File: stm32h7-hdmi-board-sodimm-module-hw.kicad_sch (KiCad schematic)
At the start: 8 parts

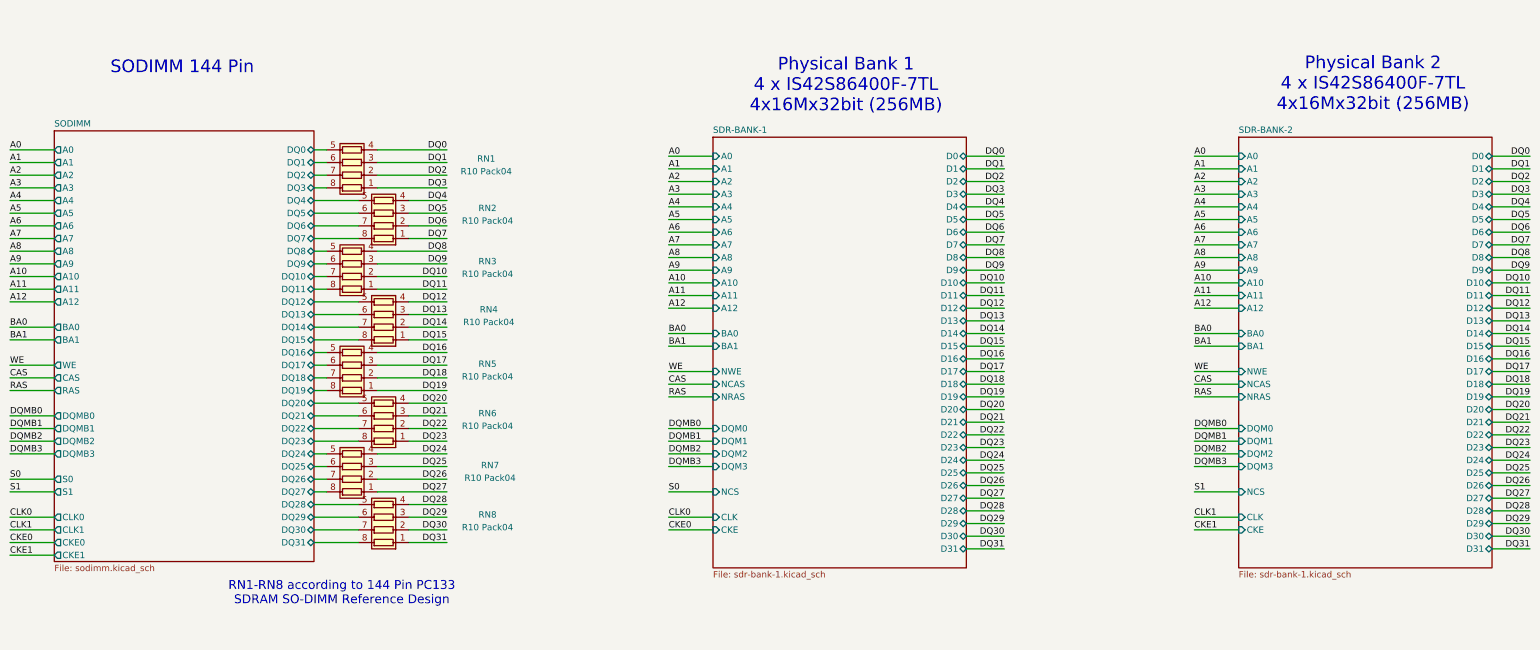
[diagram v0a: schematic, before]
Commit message: [#100470] Update schematic
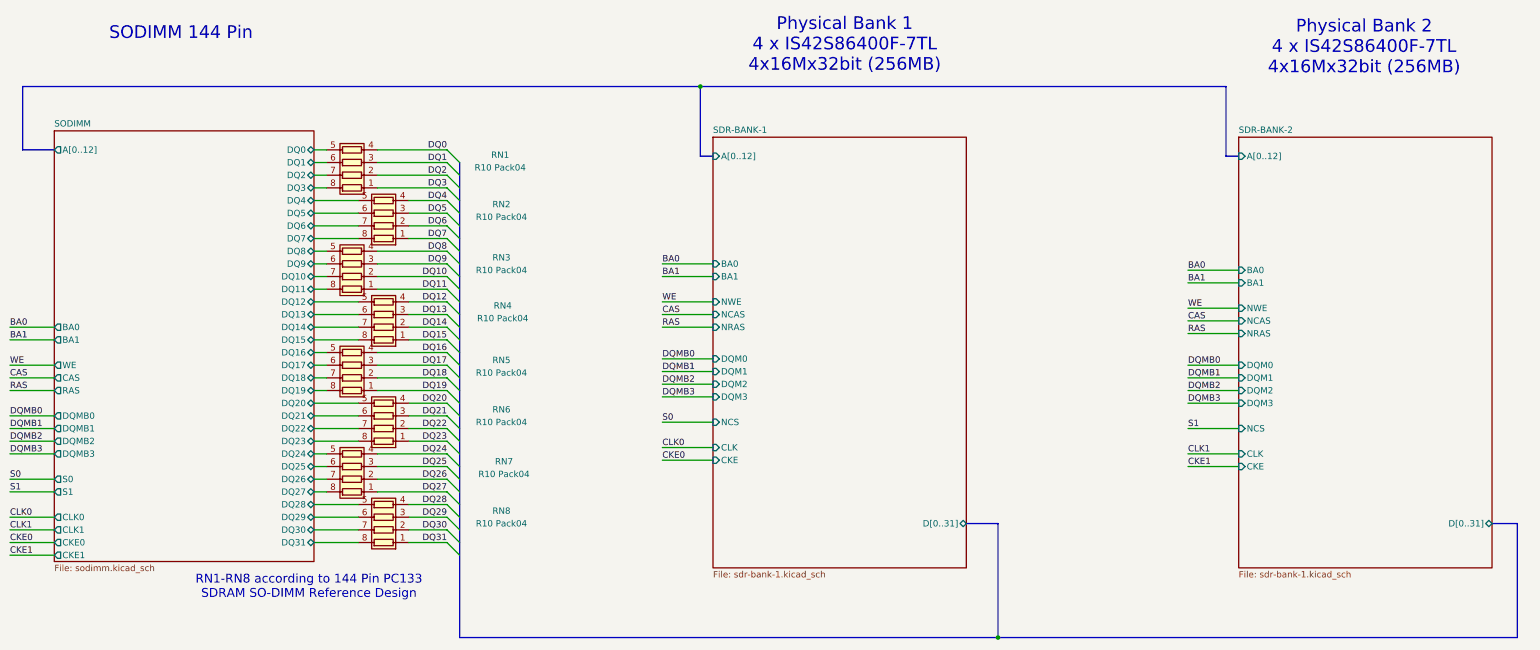
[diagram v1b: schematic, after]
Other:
- sheet SDR-BANK-1 ports: added A[0..12], D[0..31]; removed A0, A1, A10, A11, A12, A2, A3, A4, A5, A6, A7, A8, A9, D0, D1, D10, D11, D12, D13, D14, D15, D16, D17, D18, D19, D2, D20, D21, D22, D23, D24, D25, D26, D27, D28, D29, D3, D30, D31, D4, D5, D6, D7, D8, D9
- sheet SDR-BANK-2 ports: added A[0..12], D[0..31]; removed A0, A1, A10, A11, A12, A2, A3, A4, A5, A6, A7, A8, A9, D0, D1, D10, D11, D12, D13, D14, D15, D16, D17, D18, D19, D2, D20, D21, D22, D23, D24, D25, D26, D27, D28, D29, D3, D30, D31, D4, D5, D6, D7, D8, D9
- sheet SODIMM ports: added A[0..12]; removed A0, A1, A10, A11, A12, A2, A3, A4, A5, A6, A7, A8, A9
